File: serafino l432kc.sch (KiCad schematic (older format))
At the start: 23 parts

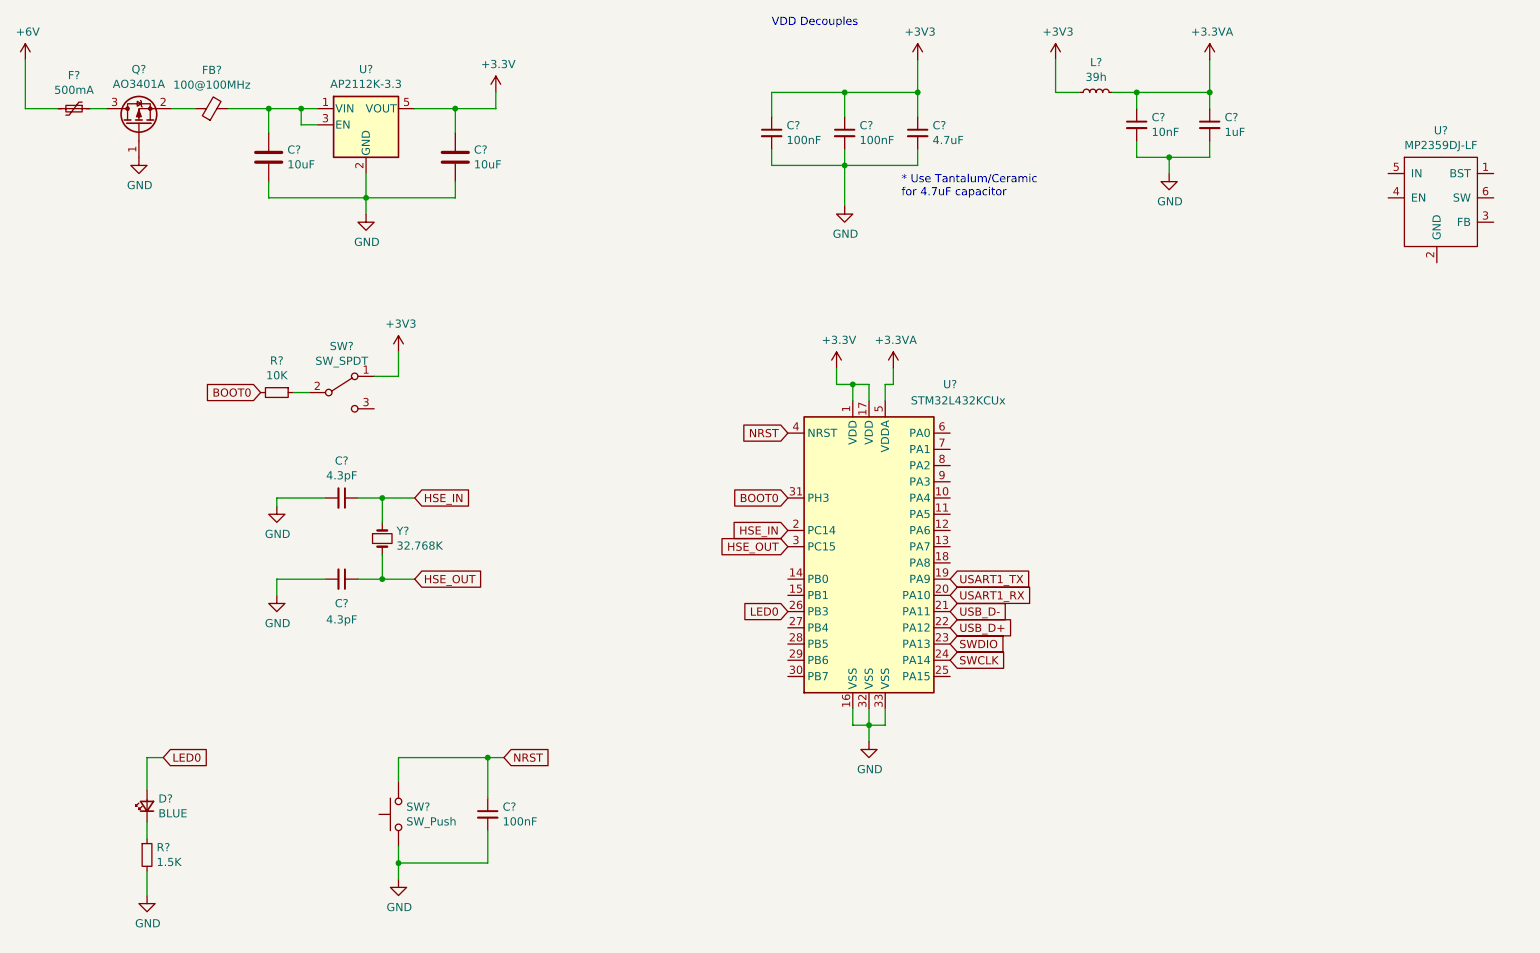
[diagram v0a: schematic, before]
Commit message: avances...
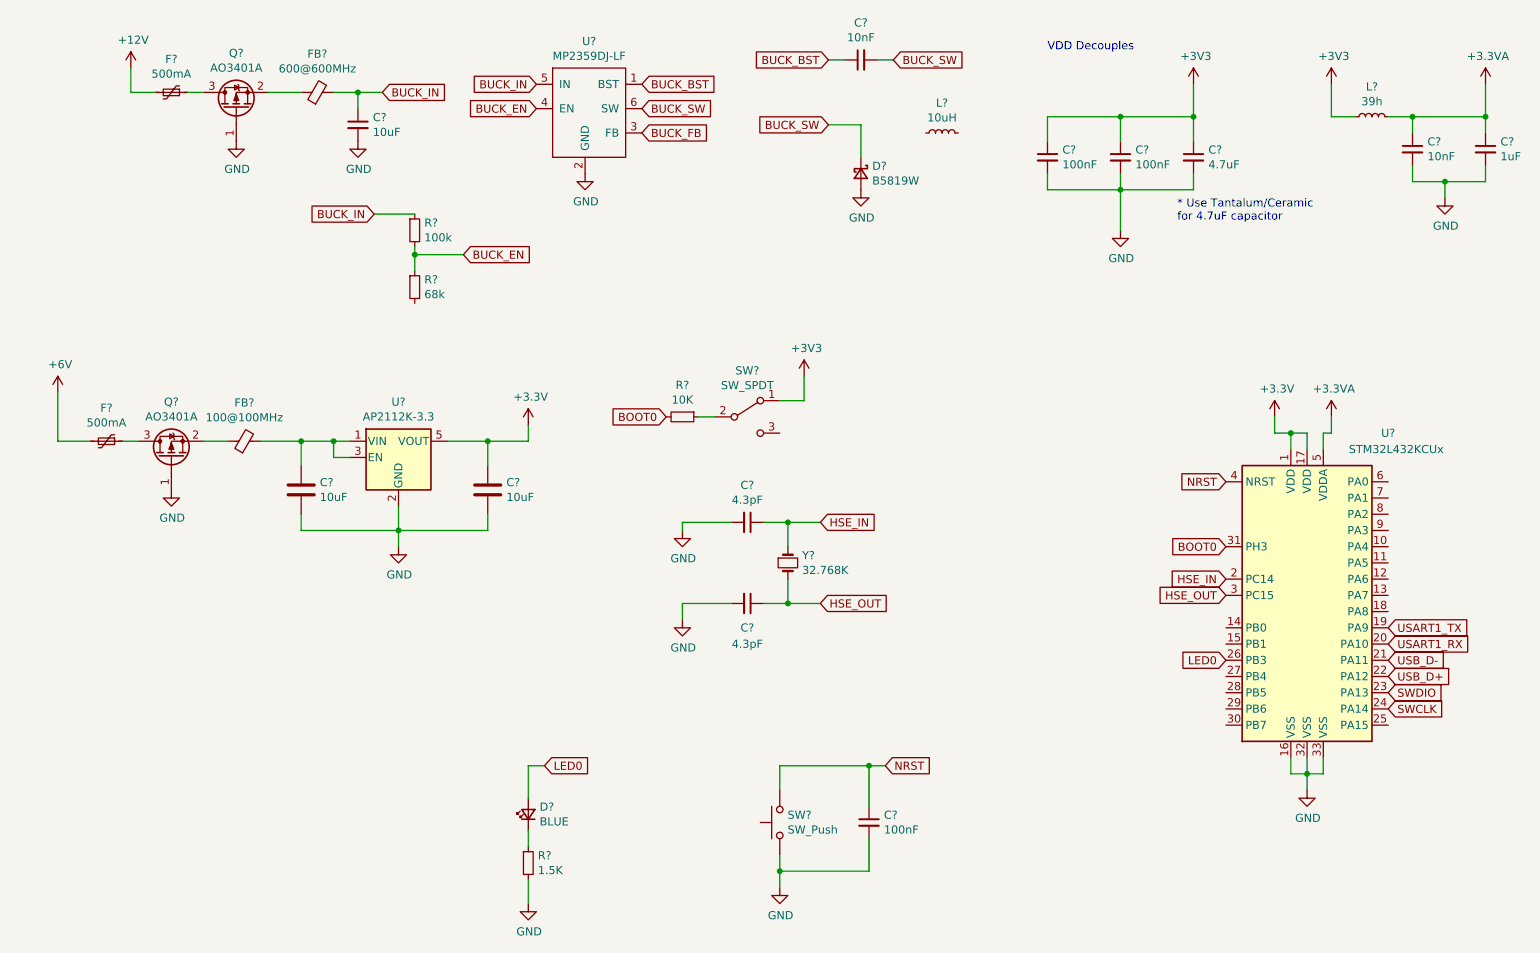
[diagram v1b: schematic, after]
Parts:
- added C?: 10uF, symbol Device:C_Small
- added C?: 10nF, symbol Device:C_Small
- added D?: B5819W, symbol Device:D_Schottky_Small
- added F?: 500mA, symbol Device:Polyfuse_Small
- added FB?: 600@600MHz, symbol Device:Ferrite_Bead_Small
- added L?: 10uH, symbol Device:L_Small
- added Q?: AO3401A, Package_TO_SOT_SMD:SOT-23, symbol Transistor_FET:AO3401A
- added R?: 100k, symbol Device:R_Small
- added R?: 68k, symbol Device:R_Small
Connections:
- net GND: now also U?.2 (GND), C?.2, D?.2 (A), Q?.1 (G)
- net BUCK_BST: now reaches U?.1 (BST)
- net BUCK_BST: now also C?.1
- net BUCK_FB: now reaches U?.3 (FB)
- net BUCK_EN: now reaches U?.4 (EN)
- net BUCK_EN: now also R?.1, R?.2
- net BUCK_IN: now reaches U?.5 (IN)
- net BUCK_IN: now also C?.1, FB?.2, R?.1
- net BUCK_SW: now reaches U?.6 (SW)
- net BUCK_SW: now also C?.2, D?.1 (K)
- new net: F?.1, Q?.3 (D)
- new net: FB?.1, Q?.2 (S)
- new net +12V: F?.2
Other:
- moved on the sheet: C?, D?, F?, FB?, L?, Q?, R?, SW?, U?, Y?
